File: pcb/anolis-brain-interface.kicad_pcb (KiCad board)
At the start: 2 copper layers, 14 x 18 mm, 27 parts, among them J1 214721-0020, SW1 EVQ-P7A01P, U1 RHD2216, U2 Setebos-I, U3 TPS70933, U4 LTC4054ES5-4.2

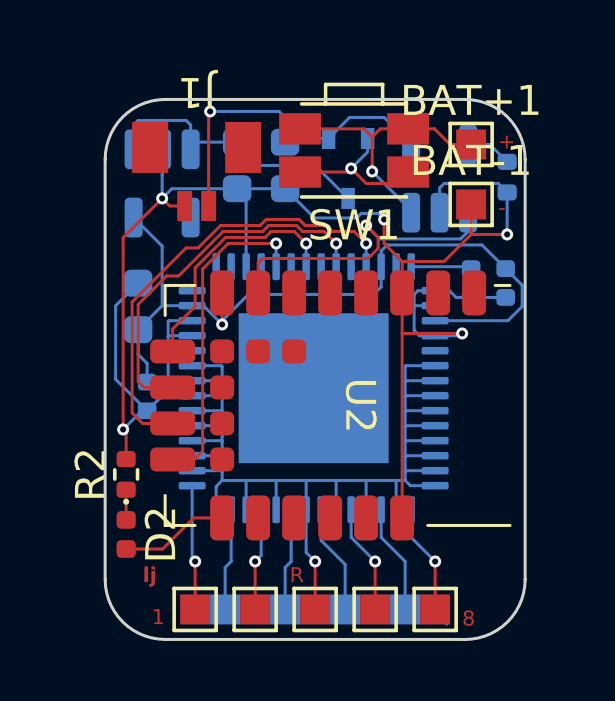
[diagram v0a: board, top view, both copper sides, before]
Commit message: Improved routing.
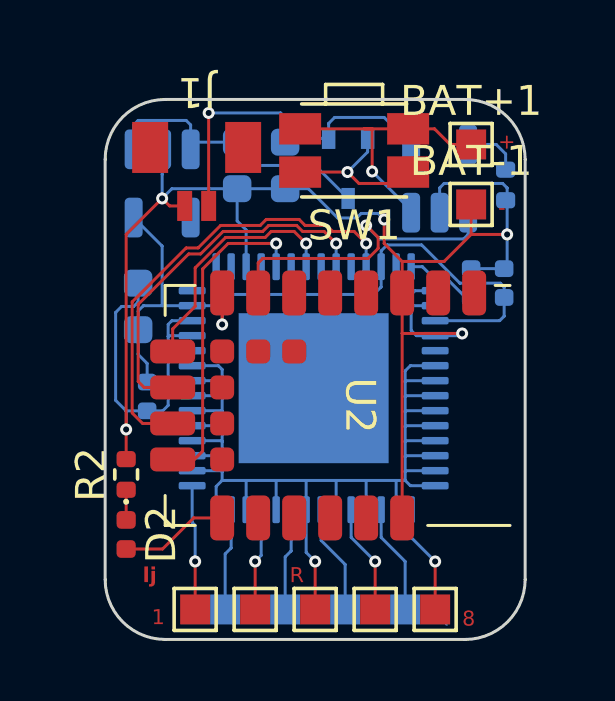
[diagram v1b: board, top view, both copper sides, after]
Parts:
- moved R1 0.26 mm to (139.3, 83.8)
- turned C6 to 90 degrees
- turned C5 to 90 degrees
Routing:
- net /GND: track 62.7 -> 63.6 mm
